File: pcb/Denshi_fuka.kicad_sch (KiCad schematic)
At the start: 51 parts, among them J1 SCREW TERMINAL, J10 Conn_01x02_Socket, J11 SCREW TERMINAL, J2 SCREW TERMINAL, J3 Digital/PWM, J4 SCREW TERMINAL, J5 Power, J6 SCREW TERMINAL, J7 Conn_01x02_Socket, J8 Analog, J9 Digital/PWM, Q1 2SK3176, Q2 2SK3176, U1 LEG_3V3, U2 LM358, U3 MCP6002-xP, U4 Si8651, U5 MCP3564R, U6 MCP4822

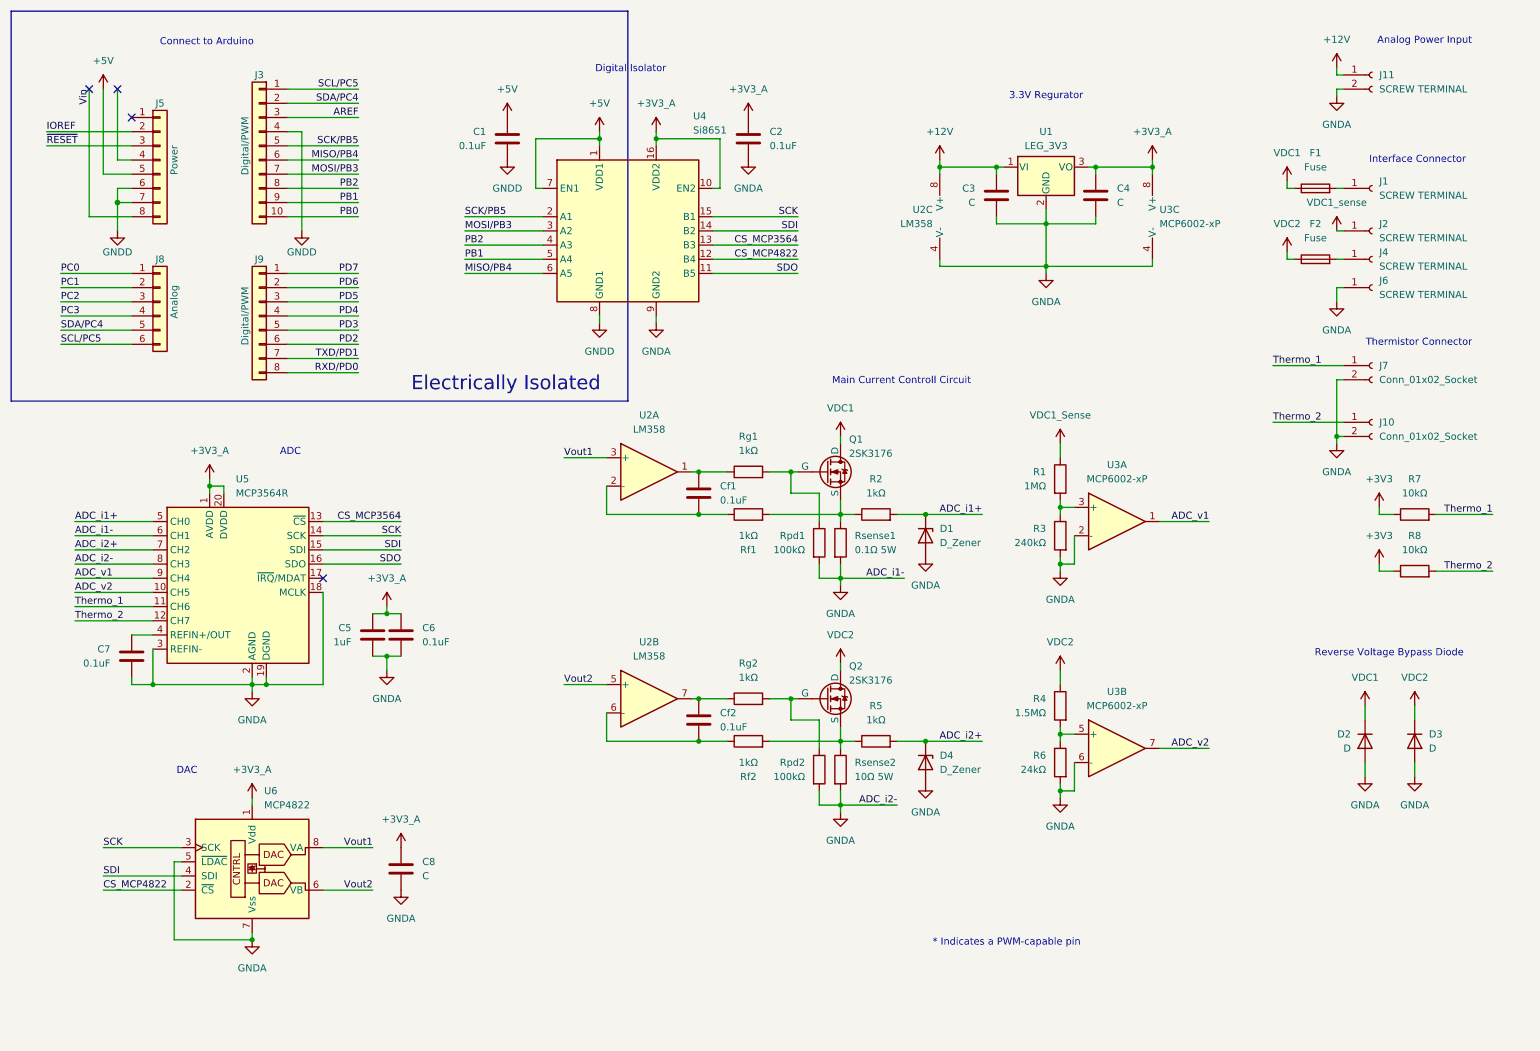
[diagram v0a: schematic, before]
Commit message: add some circuit
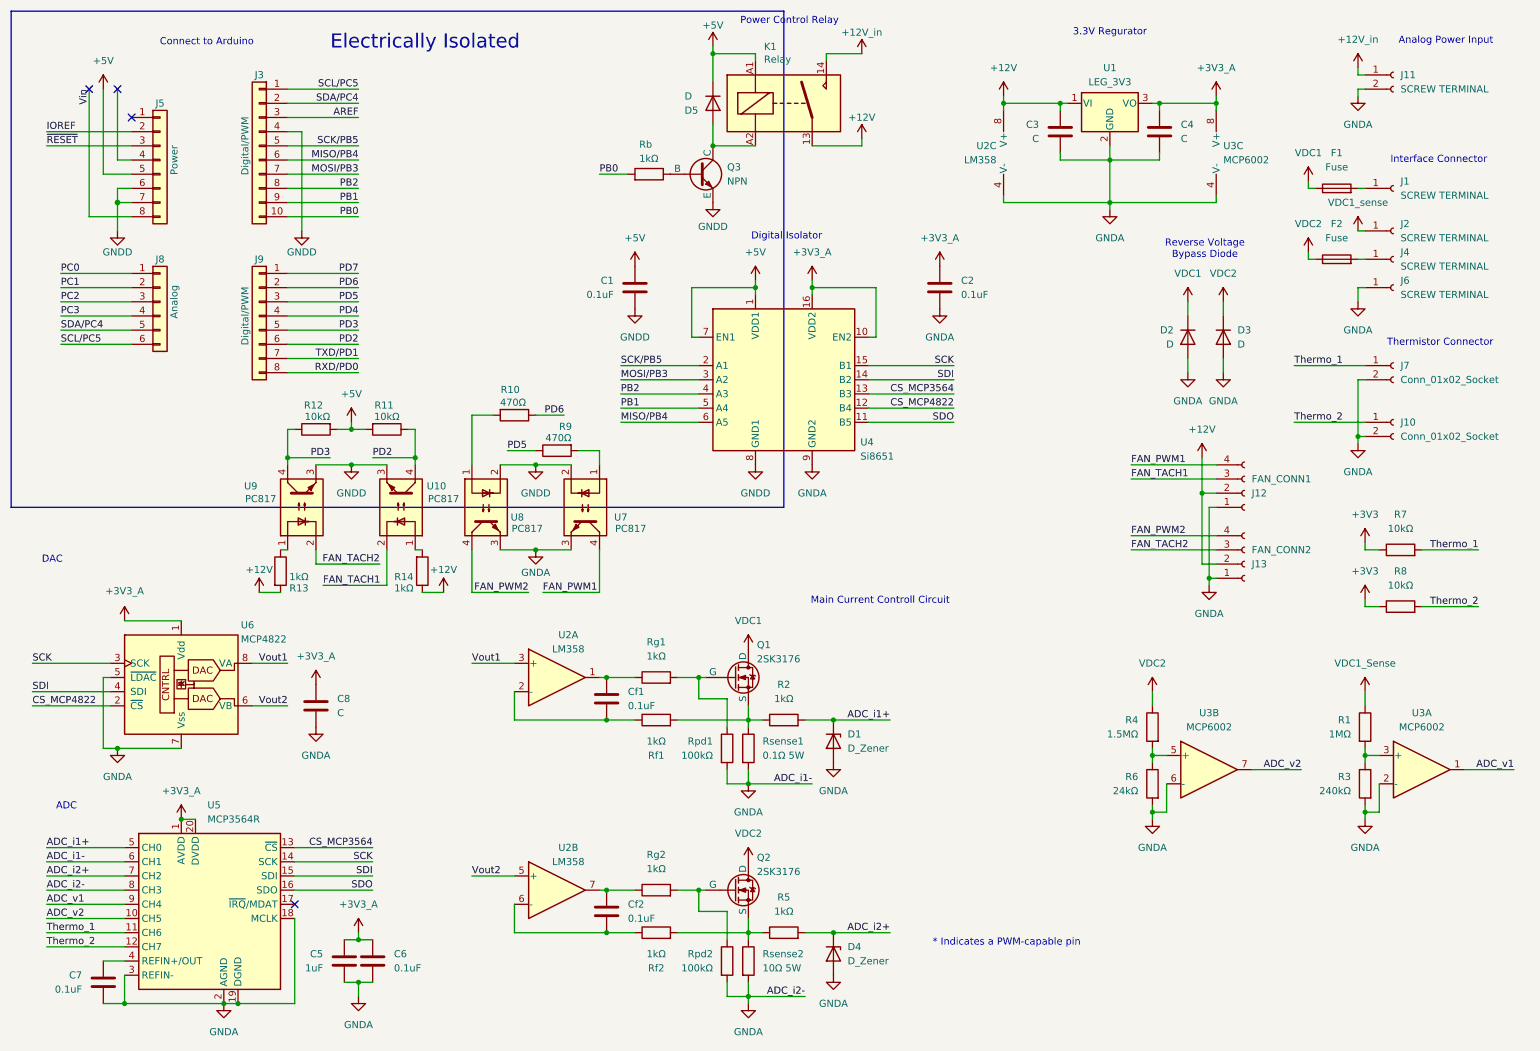
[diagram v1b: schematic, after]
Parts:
- added D5: D, symbol Device:D
- added J12: FAN_CONN1, symbol Connector:Conn_01x04_Socket
- added J13: FAN_CONN2, symbol Connector:Conn_01x04_Socket
- added K1: Relay, symbol Relay:Relay_SPST-NO
- added Q3: NPN, symbol Simulation_SPICE:NPN
- added R10, R9: 470Ω, symbol Device:R
- added R11, R12: 10kΩ, symbol Device:R
- added R13, R14, Rb: 1kΩ, symbol Device:R
- added U10, U7, U8, U9: PC817, symbol Isolator:Optocoupler_DC_PhotoNPN_AKEC
- U3: value MCP6002-xP -> MCP6002
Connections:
- net +12V: now also J12.2 (Pin_2), J13.2 (Pin_2), K1.13, R13.2, R14.1; no longer J11.1 (Pin_1)
- net +5V: now also D5.1 (K), K1.A1, R11.2, R12.2
- net GNDA: now also J12.1 (Pin_1), J13.1 (Pin_1), U7.3, U8.3
- net GNDD: now also Q3.3 (E), U10.3, U7.2, U8.2, U9.3
- net PB0: now also Rb.2
- net PD2: now also R11.1, U10.4
- net PD3: now also R12.1, U9.4
- net PD5: now also R9.1
- net PD6: now also R10.1
- new net: R9.2, U7.1
- new net: R13.1, U9.1
- new net: D5.2 (A), K1.A2, Q3.1 (C)
- new net: Q3.2 (B), Rb.1
- new net: R10.2, U8.1
- new net: R14.2, U10.1
- new net +12V_in: J11.1 (Pin_1), K1.14
- new net FAN_PWM1: J12.4 (Pin_4), U7.4
- new net FAN_PWM2: J13.4 (Pin_4), U8.4
- new net FAN_TACH1: J12.3 (Pin_3), U10.2
- new net FAN_TACH2: J13.3 (Pin_3), U9.2
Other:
- note added: "Power Control Relay"
- moved on the sheet: C1, C2, C3, C4, C5, C6, C7, C8, Cf1, Cf2, D1, D2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

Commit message: Fuck
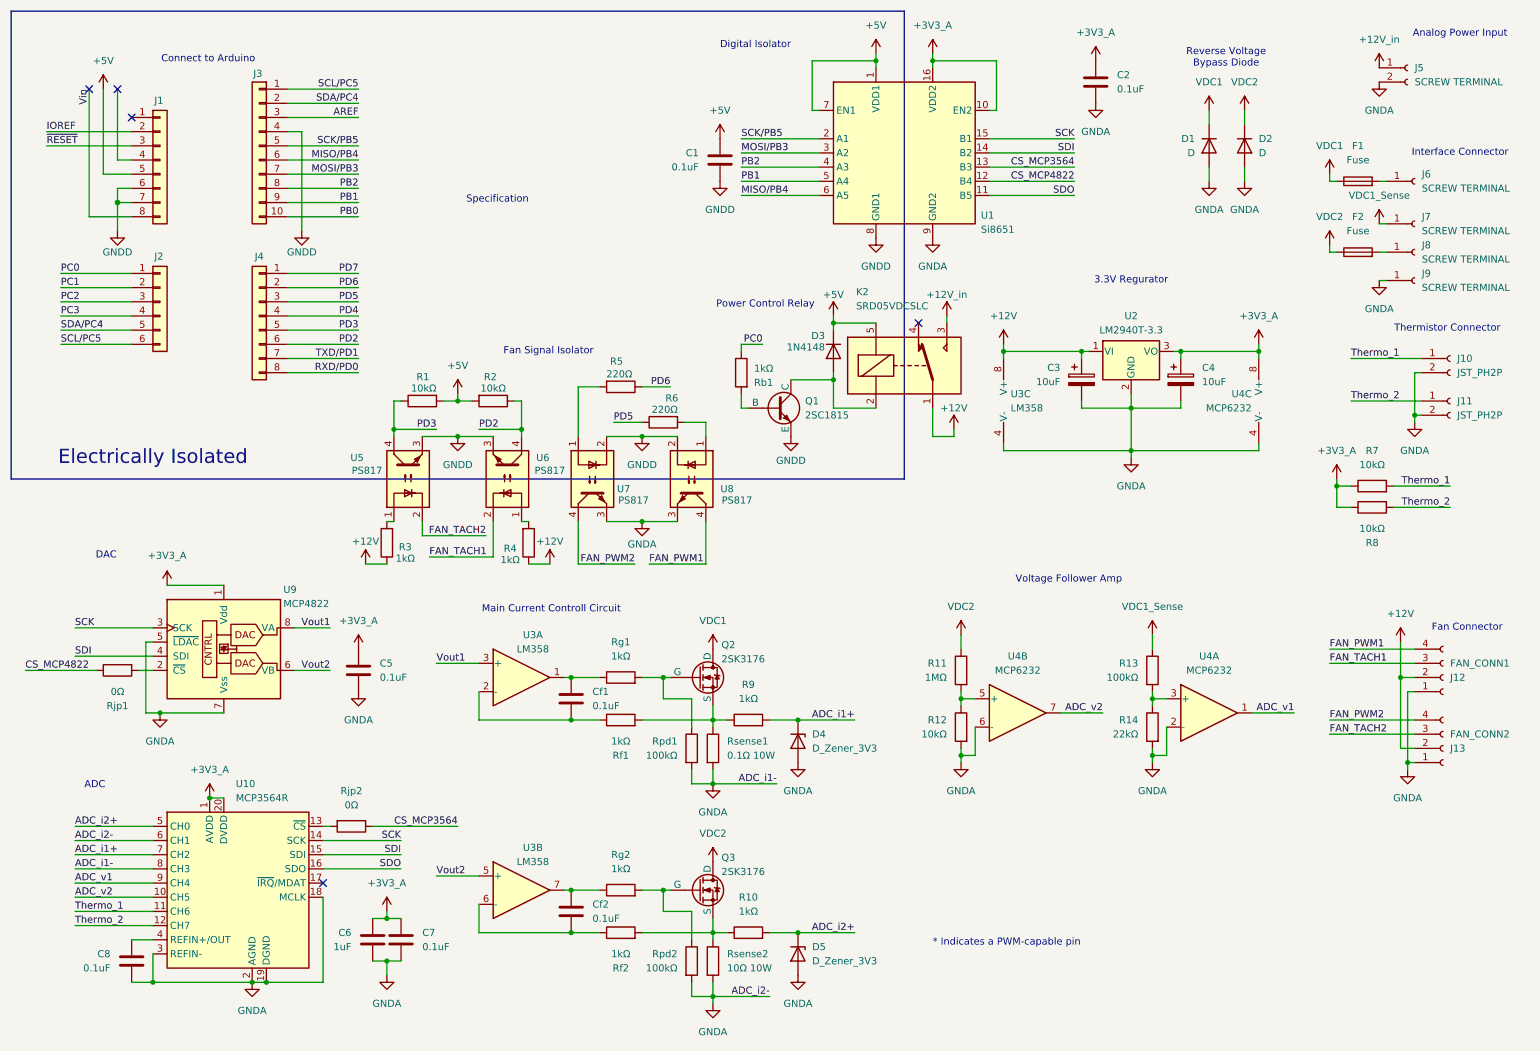
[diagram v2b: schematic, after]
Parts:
- removed C3, C4: C, symbol Device:C
- removed J5: Power, Connector_PinSocket_2.54mm:PinSocket_1x08_P2.54mm_Vertical, symbol Connector_Generic:Conn_01x08
- removed J8: Analog, Connector_PinSocket_2.54mm:PinSocket_1x06_P2.54mm_Vertical, symbol Connector_Generic:Conn_01x06
- removed J9: Digital/PWM, Connector_PinSocket_2.54mm:PinSocket_1x08_P2.54mm_Vertical, symbol Connector_Generic:Conn_01x08
- removed K1: Relay, symbol Relay:Relay_SPST-NO
- added C3, C4: 10uF, Capacitor_THT:CP_Radial_D5.0mm_P2.00mm, symbol Device:C_Polarized
- added J1, J4: Conn_01x08, Connector_PinHeader_2.54mm:PinHeader_1x08_P2.54mm_Vertical, symbol Connector_Generic:Conn_01x08
- added J2: Conn_01x06, Connector_PinHeader_2.54mm:PinHeader_1x06_P2.54mm_Vertical, symbol Connector_Generic:Conn_01x06
- added K2: SRD05VDCSLC, Relay_THT:Relay_SPDT_SANYOU_SRD_Series_Form_C, symbol Relay:SANYOU_SRD_Form_C
- added Rjp1, Rjp2: 0Ω, Resistor_THT:R_Axial_DIN0309_L9.0mm_D3.2mm_P12.70mm_Horizontal, symbol Device:R
- C5: renamed from C8; value C -> 0.1uF; footprint (none) -> Capacitor_THT:C_Disc_D5.0mm_W2.5mm_P5.00mm
- C6: renamed from C5; footprint Capacitor_THT:C_Disc_D5.0mm_W2.5mm_P5.00mm -> Capacitor_THT:C_Disc_D3.0mm_W1.6mm_P2.50mm
- D3: renamed from D5; value D -> 1N4148; footprint (none) -> Diode_THT:D_DO-35_SOD27_P7.62mm_Horizontal
- D4: renamed from D1; value D_Zener -> D_Zener_3V3; footprint (none) -> Diode_THT:D_DO-35_SOD27_P7.62mm_Horizontal
- D5: renamed from D4; value D_Zener -> D_Zener_3V3; footprint (none) -> Diode_THT:D_DO-35_SOD27_P7.62mm_Horizontal
- F1, F2: footprint (none) -> MyParts:MF-563
- J10: renamed from J7; value Conn_01x02_Socket -> JST_PH2P; footprint (none) -> Connector_JST:JST_PH_B2B-PH-K_1x02_P2.00mm_Vertical
- J11: renamed from J10; value Conn_01x02_Socket -> JST_PH2P; footprint (none) -> Connector_JST:JST_PH_B2B-PH-K_1x02_P2.00mm_Vertical
- J12, J13: footprint (none) -> Connector:FanPinHeader_1x04_P2.54mm_Vertical
- J3: value Digital/PWM -> Conn_01x10; footprint Connector_PinSocket_2.54mm:PinSocket_1x10_P2.54mm_Vertical -> Connector_PinHeader_2.54mm:PinHeader_1x10_P2.54mm_Vertical
- J5: renamed from J11; footprint (none) -> TerminalBlock_Phoenix:TerminalBlock_Phoenix_PT-1,5-2-5.0-H_1x02_P5.00mm_Horizontal
- J6: renamed from J1; footprint (none) -> Aki-Parts:PCB-20
- J7: renamed from J2; footprint (none) -> Aki-Parts:PCB-20
- J8: renamed from J4; footprint (none) -> Aki-Parts:PCB-20
- J9: renamed from J6; footprint (none) -> Aki-Parts:PCB-20
- Q1: renamed from Q3; value NPN -> 2SC1815; footprint (none) -> Package_TO_SOT_THT:TO-92_Inline
- R1: renamed from R12; footprint (none) -> Resistor_THT:R_Axial_DIN0207_L6.3mm_D2.5mm_P10.16mm_Horizontal
- R10: renamed from R5; footprint (none) -> Resistor_THT:R_Axial_DIN0207_L6.3mm_D2.5mm_P10.16mm_Horizontal
- R11: renamed from R4; value 1.5MΩ -> 1MΩ
- R12: renamed from R6; value 24kΩ -> 10kΩ
- R13: renamed from R1; value 1MΩ -> 100kΩ
- R14: renamed from R3; value 240kΩ -> 22kΩ
- R2: renamed from R11; footprint (none) -> Resistor_THT:R_Axial_DIN0207_L6.3mm_D2.5mm_P10.16mm_Horizontal
- R3: renamed from R13; footprint (none) -> Resistor_THT:R_Axial_DIN0207_L6.3mm_D2.5mm_P10.16mm_Horizontal
- R4: renamed from R14; footprint (none) -> Resistor_THT:R_Axial_DIN0207_L6.3mm_D2.5mm_P10.16mm_Horizontal
- R5: renamed from R10; value 470Ω -> 220Ω; footprint (none) -> Resistor_THT:R_Axial_DIN0207_L6.3mm_D2.5mm_P10.16mm_Horizontal
- R6: renamed from R9; value 470Ω -> 220Ω; footprint (none) -> Resistor_THT:R_Axial_DIN0207_L6.3mm_D2.5mm_P10.16mm_Horizontal
- R7, R8, Rpd1, Rpd2: footprint (none) -> Resistor_THT:R_Axial_DIN0207_L6.3mm_D2.5mm_P10.16mm_Horizontal
- R9: renamed from R2; footprint (none) -> Resistor_THT:R_Axial_DIN0207_L6.3mm_D2.5mm_P10.16mm_Horizontal
- Rb1: renamed from Rb; footprint (none) -> Resistor_THT:R_Axial_DIN0207_L6.3mm_D2.5mm_P10.16mm_Horizontal
- Rf1, Rf2, Rg1, Rg2: footprint Resistor_THT:R_Axial_DIN0207_L6.3mm_D2.5mm_P10.16mm_Horizontal -> Resistor_THT:R_Axial_DIN0309_L9.0mm_D3.2mm_P12.70mm_Horizontal
- Rsense1: value 0.1Ω 5W -> 0.1Ω 10W
- Rsense2: value 10Ω 5W -> 10Ω 10W
- U1: renamed from U4; footprint (none) -> MyParts:DIP-16_W15.24mm (600mil)
- U10: renamed from U5; footprint (none) -> MyParts:DIP-20_W15.24mm_Socket_LongPads
- U2: renamed from U1; value LEG_3V3 -> LM2940T-3.3
- U4: renamed from U3; value MCP6002 -> MCP6232
- U5: renamed from U9; value PC817 -> PS817; footprint (none) -> Package_DIP:DIP-4_W7.62mm_LongPads
- U6: renamed from U10; value PC817 -> PS817; footprint (none) -> Package_DIP:DIP-4_W7.62mm_LongPads
- U7: renamed from U8; value PC817 -> PS817; footprint (none) -> Package_DIP:DIP-4_W7.62mm_LongPads
- U8: renamed from U7; value PC817 -> PS817; footprint (none) -> Package_DIP:DIP-4_W7.62mm_LongPads
- renumbered C6 to C7, C7 to C8, D2 to D1, D3 to D2, Q1 to Q2, Q2 to Q3, U2 to U3, U6 to U9
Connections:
- net +3V3 is gone; now on net +3V3_A: R7.1, R8.1
- net VDC1_sense is gone; now on net VDC1_Sense: J7.1 (Pin_1)
- net +12V: now also R3.1, C3.1, K2.1; no longer R3.2
- net +12V_in: now also K2.3
- net +3V3_A: now also C4.1
- net +5V: now also J1.5 (Pin_5), K2.5
- net ADC_i1+: now also U10.7 (CH2); no longer U10.5 (CH0)
- net ADC_i2+: now also U10.5 (CH0); no longer U10.7 (CH2)
- net CS_MCP3564: now also Rjp2.1; no longer U10.13 (~{CS})
- net CS_MCP4822: now also Rjp1.1; no longer U9.2 (~{CS})
- net GNDA: now also C3.2, C4.2
- net GNDD: now also J1.6 (Pin_6), J1.7 (Pin_7)
- net IOREF: now also J1.2 (Pin_2)
- net PB0: no longer Rb1.2
- net PC0: now also Rb1.1, J2.1 (Pin_1)
- net PC1: now also J2.2 (Pin_2)
- net PC2: now also J2.3 (Pin_3)
- net PC3: now also J2.4 (Pin_4)
- net PD2: now also J4.6 (Pin_6)
- net PD3: now also J4.5 (Pin_5)
- net PD4: now also J4.4 (Pin_4)
- net PD5: now also J4.3 (Pin_3)
- net PD6: now also J4.2 (Pin_2)
- net PD7: now also J4.1 (Pin_1)
- net RXD/PD0: now also J4.8 (Pin_8)
- net SCL/PC5: now also J2.6 (Pin_6)
- net SDA/PC4: now also J2.5 (Pin_5)
- net TXD/PD1: now also J4.7 (Pin_7)
- net VDC1: now also Q2.2 (D); no longer Q2.1 (D)
- net VDC2: now also Q3.2 (D); no longer Q3.1 (D)
- net Vin: now also J1.8 (Pin_8)
- net ~{RESET}: now also J1.3 (Pin_3)
- net at U5.1: now also R3.2; no longer R3.1
- net at D3.2 (A), Q1.1 (C): now also K2.2
- net at Rg2.2, Rpd2.1: now also Q3.1 (G); no longer Q3.2 (G)
- net at Q1.2 (B): now also Rb1.2; no longer Rb1.1
- net at Rg1.2, Rpd1.1: now also Q2.1 (G); no longer Q2.2 (G)
- new net: Rjp1.2, U9.2 (~{CS})
- new net: Rjp2.2, U10.13 (~{CS})
- no-connect marks 4 -> 5
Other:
- note added: "Fan Connector"
- note added: "Fan Signal Isolator"
- note added: "Specification"
- note added: "Voltage Follower Amp"
- moved on the sheet: C1, C2, C5, C6, C7, C8, Cf1, Cf2, D1, D2, D3, D4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
